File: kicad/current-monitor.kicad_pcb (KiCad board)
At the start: 2 copper layers, 55.2 x 21 mm, 29 parts, among them J1 Conn_01x02_Male, J2 Conn_01x02_Male, J3 Conn_02x05_Top_Bottom, U1 SIT1602BI-21-XXE-8.192000G, U2 MIC5504-3.3YM5

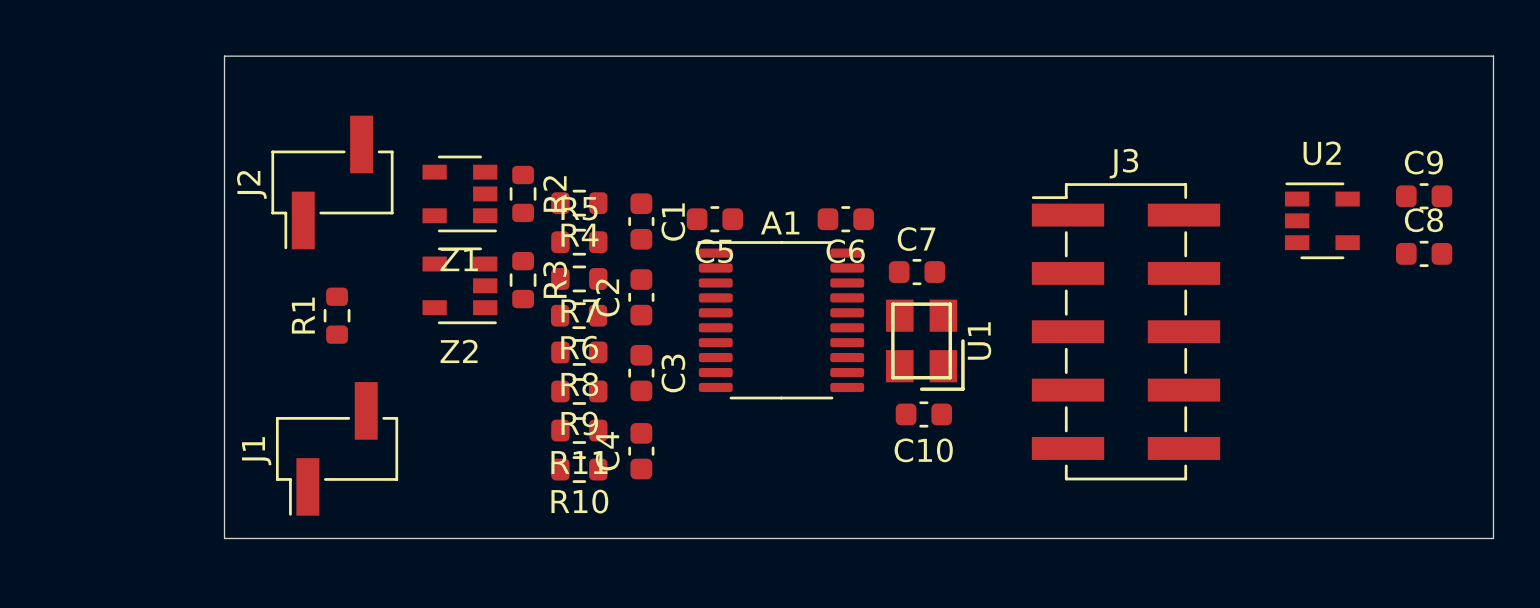
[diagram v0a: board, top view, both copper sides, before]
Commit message: snapshot
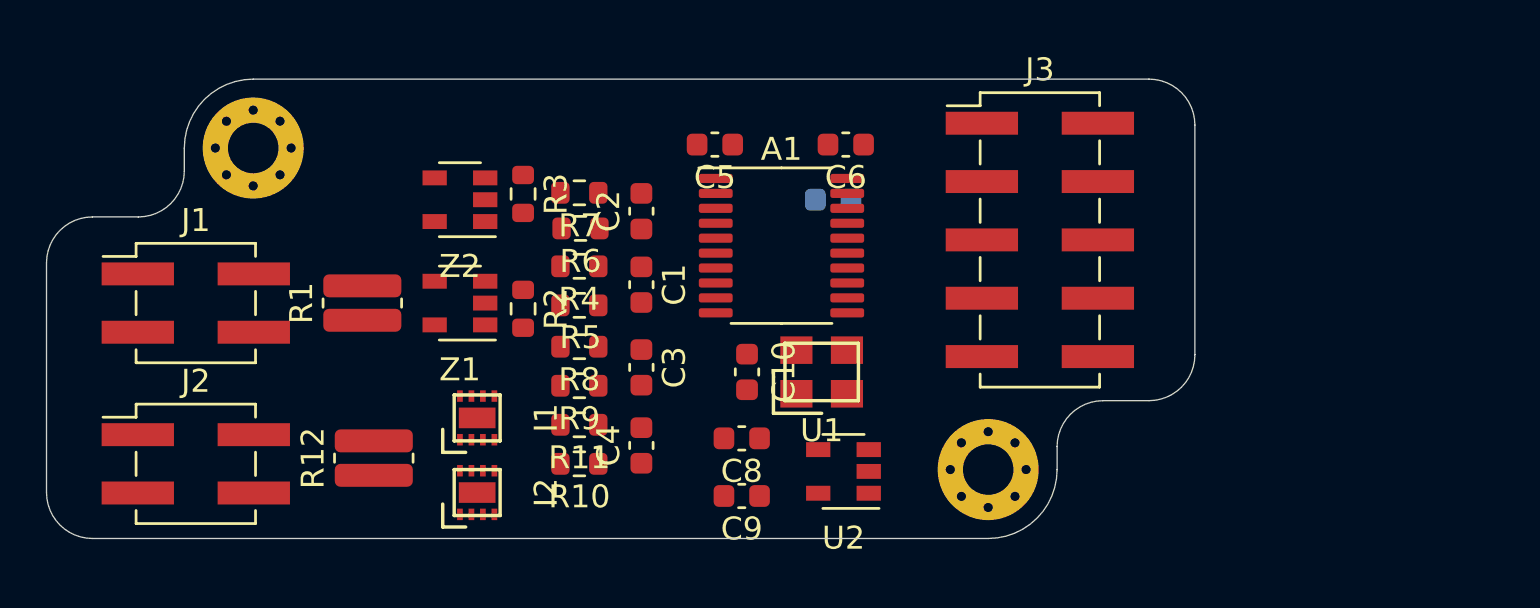
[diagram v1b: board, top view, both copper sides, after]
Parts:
- added H1: MountingHole, MountingHole:MountingHole_2.2mm_M2_Pad_Via, F.Cu at (142.0, 103.0)
- added H2: MountingHole, MountingHole:MountingHole_2.2mm_M2_Pad_Via, F.Cu at (174.0, 117.0)
- added I1: INA381, HH_TexasInstruments:INA381-WSON, F.Cu at (151.8, 114.8)
- added I2: INA381, HH_TexasInstruments:INA381-WSON, F.Cu at (151.8, 118.0)
- added R12: 2, Resistor_SMD:R_0612_1632Metric, F.Cu at (147.2, 116.5)
- C7: moved to B.Cu
- J1, J2: value Conn_01x02_Male -> Conn_02x02_Odd_Even; footprint Connector_PinHeader_2.54mm:PinHeader_1x02_P2.54mm_Vertical_SMD_Pin1Left -> Connector_PinHeader_2.54mm:PinHeader_2x02_P2.54mm_Vertical_SMD
- J3: value Conn_02x05_Top_Bottom -> Conn_02x05_Odd_Even
- R1: footprint Resistor_SMD:R_0603_1608Metric -> Resistor_SMD:R_0612_1632Metric
- moved C9 32.4 mm to (163.3, 118.2), turned to 180 degrees
- moved C8 30.8 mm to (163.3, 115.6), turned to 180 degrees
- moved U2 23.5 mm to (167.7, 117.1), turned to 180 degrees
- moved J2 13.6 mm to (139.5, 116.8), turned to 0 degrees
- moved J1 8.84 mm to (139.5, 109.8), turned to 0 degrees
- moved C10 7.92 mm to (163.5, 112.8), turned to 90 degrees
- moved J3 5.48 mm to (176.2, 107.0)
- moved R2 5.00 mm to (153.8, 110.0)
- moved C7 4.82 mm to (167.2, 105.2), turned to 0 degrees
- moved Z1 4.75 mm to (151.0, 109.8)
- moved U1 4.55 mm to (166.8, 112.8), turned to 0 degrees
- moved R6 3.80 mm to (156.2, 106.5)
- moved C2 3.75 mm to (158.9, 105.8)
- moved R3 3.75 mm to (153.8, 105.0)
- moved R7 3.75 mm to (156.2, 105.0)
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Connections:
- J1 pad 1: /sensors/S1- -> GND
- J1 pad 2: GND -> /sensors/S1-
- J2 pad 1: /sensors/S1+ -> GND
- J2 pad 2: GND -> /sensors/S3-
- J3 pad 2: /adc/CIPO -> /adc/GND
- J3 pad 3: /adc/SCLK -> /adc/CIPO
- J3 pad 4: /adc/~CS -> /power/5V
- J3 pad 5: /adc/~DRDY -> /adc/SCLK
- J3 pad 6: /adc/GND -> /adc/3V3
- J3 pad 7: /power/5V -> /adc/~CS
- J3 pad 8: /adc/3V3 -> /adc/GND
- J3 pad 9: /adc/GND -> /adc/~DRDY
- R1 pad 1: /sensors/S1- -> /sensors/S1+
- R1 pad 2: /sensors/S1+ -> /sensors/S1-
- R10 pad 2: (no net) -> /sensors/OUT4
- R4 pad 2: /sensors/OUT1 -> (no net)
- R6 pad 2: /sensors/OUT2 -> (no net)
- R8 pad 2: (no net) -> /sensors/OUT3
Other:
- board size 55.2 x 21 mm -> 50 x 20 mm
